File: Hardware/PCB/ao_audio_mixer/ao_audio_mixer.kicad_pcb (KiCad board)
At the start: 2 copper layers, 66 x 170 mm, 15 parts, among them J1 AudioJack2, J2 AudioJack2, J3 AudioJack2, J4 Conn_01x08, J5 AudioJack2, J6 AudioJack2

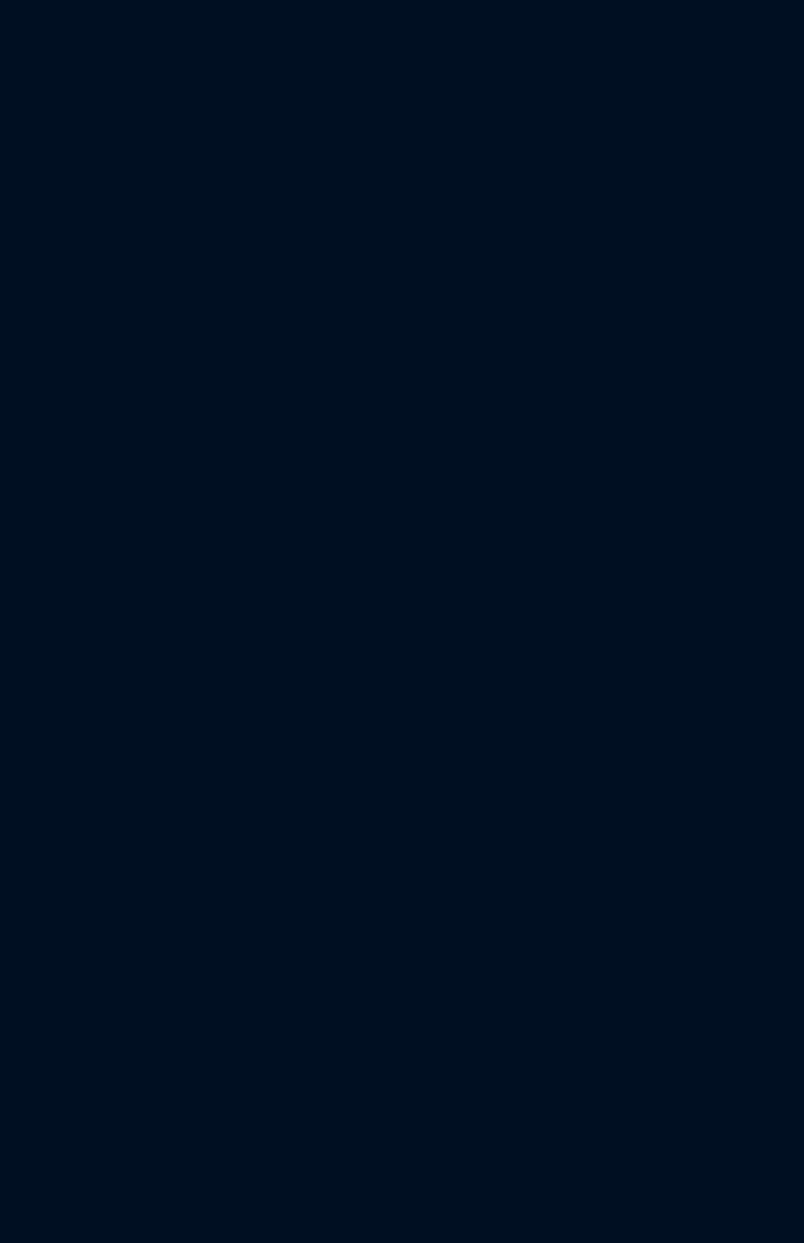
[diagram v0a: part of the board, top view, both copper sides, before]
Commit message: Restore deleted board
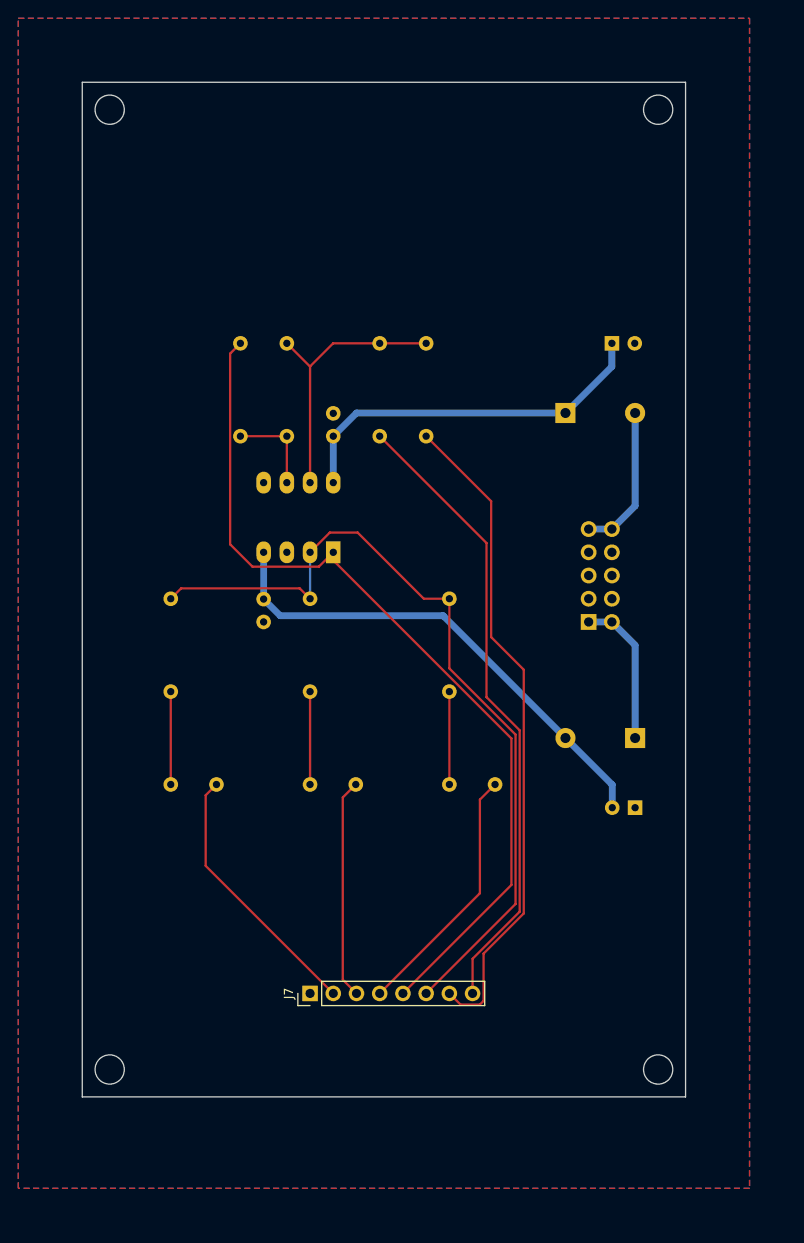
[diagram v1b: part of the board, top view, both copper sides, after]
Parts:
- added C1: 1uF, ao_tht:C_Rect_L7.2mm_W7.2mm_P5.00mm_FKS2_FKP2_MKS2_MKP2, B.Cu at (76.7, 112.8)
- added C2: 1uF, ao_tht:C_Rect_L7.2mm_W7.2mm_P5.00mm_FKS2_FKP2_MKS2_MKP2, B.Cu at (91.9, 112.8)
- added C3: 1uF, ao_tht:C_Rect_L7.2mm_W7.2mm_P5.00mm_FKS2_FKP2_MKS2_MKP2, B.Cu at (107.2, 112.8)
- added C4: 10uF, ao_tht:CP_Radial_D6.3mm_P2.50mm, B.Cu at (124.9, 64.6)
- added C5: 10uF, ao_tht:CP_Radial_D6.3mm_P2.50mm, B.Cu at (127.5, 115.4)
- added C6: 100nF, ao_tht:C_Disc_D3.0mm_W1.6mm_P2.50mm, B.Cu at (94.5, 74.7)
- added C7: 100nF, ao_tht:C_Disc_D3.0mm_W1.6mm_P2.50mm, B.Cu at (86.8, 95.0)
- added D1: 1N5817, ao_tht:D_DO-41_SOD81_P7.62mm_Horizontal, B.Cu at (119.9, 72.2)
- added D2: 1N5817, ao_tht:D_DO-41_SOD81_P7.62mm_Horizontal, B.Cu at (127.5, 107.7)
- added GRAF1: Panel holes, ao_audio_mixer:ao_audio_mixer_panel_slide_holes, F.Cu at (-76.1, 26.0)
- added GRAF2: AO Logo, ao_tht:analogoutput, B.Cu at (83.0, 46.0)
- added GRAF3: CC0 Logo, ao_tht:CC0_logo, B.Cu at (109.0, 54.0)
- added H1: MountingHole, ao_tht:MountingHole_3.2mm_M3, B.Cu at (70.0, 39.0)
- added H2: MountingHole, ao_tht:MountingHole_3.2mm_M3, B.Cu at (130.0, 39.0)
- added H3: MountingHole, ao_tht:MountingHole_3.2mm_M3, F.Cu at (70.0, 144.0)
- added H4: MountingHole, ao_tht:MountingHole_3.2mm_M3, F.Cu at (130.0, 144.0)
- added J7: Conn_01x08, Connector_PinHeader_2.54mm:PinHeader_1x08_P2.54mm_Vertical, F.Cu at (91.9, 135.7)
- added J8: Synth_power_2x5, ao_tht:Power_Header, B.Cu at (122.4, 95.0)
- added R1: 100k, ao_tht:R_Axial_DIN0207_L6.3mm_D2.5mm_P10.16mm_Horizontal, B.Cu at (76.7, 92.5)
- added R2: 100k, ao_tht:R_Axial_DIN0207_L6.3mm_D2.5mm_P10.16mm_Horizontal, B.Cu at (91.9, 92.5)
- added R3: 100k, ao_tht:R_Axial_DIN0207_L6.3mm_D2.5mm_P10.16mm_Horizontal, B.Cu at (107.2, 92.5)
- added R4: 10k, ao_tht:R_Axial_DIN0207_L6.3mm_D2.5mm_P10.16mm_Horizontal, B.Cu at (84.3, 74.7)
- added R5: 10k, ao_tht:R_Axial_DIN0207_L6.3mm_D2.5mm_P10.16mm_Horizontal, B.Cu at (89.4, 64.6)
- added R6: 1k, ao_tht:R_Axial_DIN0207_L6.3mm_D2.5mm_P10.16mm_Horizontal, B.Cu at (104.6, 74.7)
- added R7: 1k, ao_tht:R_Axial_DIN0207_L6.3mm_D2.5mm_P10.16mm_Horizontal, B.Cu at (99.5, 74.7)
- added U1: TL072, ao_tht:DIP-8_W7.62mm_Socket_LongPads, B.Cu at (94.5, 87.4)
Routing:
- net Net-(J7-Pad5): track 0.00 -> 96.7 mm
- net Net-(J7-Pad6): track 0.00 -> 90.6 mm
- net OUT1: track 0.00 -> 72.4 mm
- net OUT2: track 0.00 -> 69.4 mm
- net -12V: track 0.00 -> 54.2 mm
- net +12V: track 0.00 -> 41.3 mm
- net Net-(R5-Pad1): track 0.00 -> 30.1 mm
- net Net-(C1-Pad2): track 0.00 -> 29.1 mm
- net Net-(C3-Pad2): track 0.00 -> 28.1 mm
- net Net-(C2-Pad2): track 0.00 -> 24.1 mm
- net /-12_IN: track 0.00 -> 16.3 mm
- net /+12_IN: track 0.00 -> 16.3 mm
- net Net-(R4-Pad1): track 0.00 -> 10.2 mm
- net Net-(C3-Pad1): track 0.00 -> 10.2 mm
- net Net-(C2-Pad1): track 0.00 -> 10.2 mm
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- added copper zone on B.Cu, net GND
- added copper zone on F.Cu, net GND
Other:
- board size 66 x 170 mm -> 156 x 170 mm
- board text added: "Main board"
- board text added: "Rich Holmes CC0 1.0 April 2021"
- board text added: "https://github.com/holmesrichards/audiomixer"
